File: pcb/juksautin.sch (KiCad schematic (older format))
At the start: 27 parts, among them J1 Screw_Terminal_01x09, J2 Serial_Debug, J3 AVR-ISP-6, J4 Conn_01x09, U1 SP3485EN, U2 SRV05-4, U3 R-78E5.0-0.5, U4 ATmega328P-AU, Y1 X322516MLB4SI

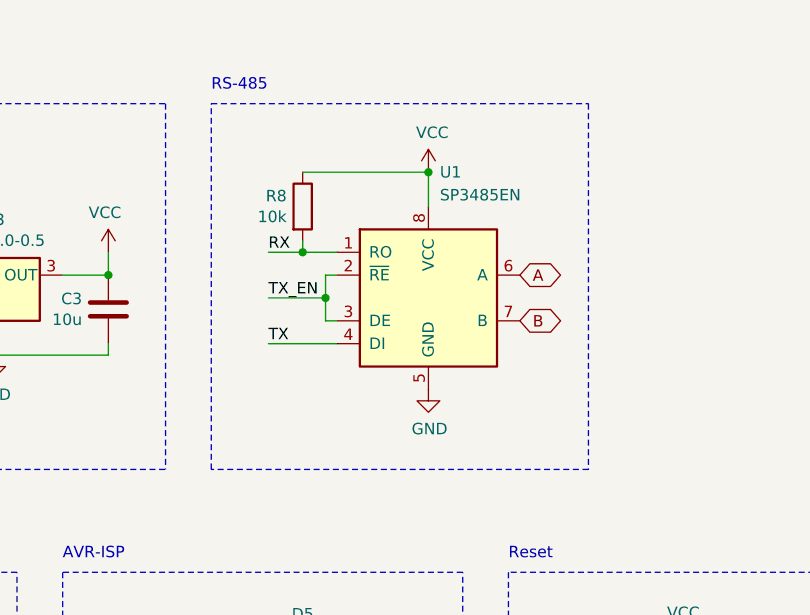
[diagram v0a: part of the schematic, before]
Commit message: pcb: Some changes. Don't remember anymore.
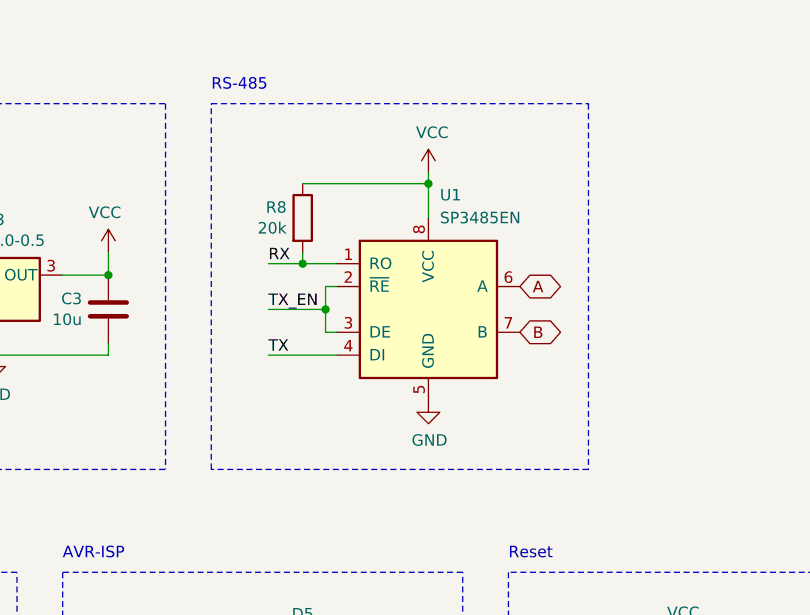
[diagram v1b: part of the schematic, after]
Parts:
- R8: value 10k -> 20k; LCSC C25804 -> C4184
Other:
- moved on the sheet: R8, U1
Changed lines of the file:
@@
 L power:GND #PWR0101
 U 1 1 60C357A5
-P 3750 2250
-F 0 "#PWR0101" H 3750 2000 50  0001 C CNN
-F 1 "GND" H 3755 2077 50  0000 C CNN
-F 2 "" H 3750 2250 50  0001 C CNN
-F 3 "" H 3750 2250 50  0001 C CNN
-	1    3750 2250
+P 3750 2300
+F 0 "#PWR0101" H 3750 2050 50  0001 C CNN
+F 1 "GND" H 3755 2127 50  0000 C CNN
+F 2 "" H 3750 2300 50  0001 C CNN
+F 3 "" H 3750 2300 50  0001 C CNN
+	1    3750 2300
 	1    0    0    -1
 $EndComp
@@
 LOW/HIGH/HI-Z\nemulates NTC
 Wire Wire Line
-	3350 1950 3300 1950
-Wire Wire Line
-	3350 1750 3300 1750
-Wire Wire Line
-	3300 1750 3300 1850
+	3350 2000 3300 2000
+Wire Wire Line
+	3350 1800 3300 1800
+Wire Wire Line
+	3300 1800 3300 1900
 Wire Wire Line
 	5650 5850 5650 5950
@@
 $EndComp
 Wire Wire Line
-	3750 1450 3750 1300
+	3750 1500 3750 1350
 $Comp
 L power:VCC #PWR0107
@@
 Text GLabel 1500 3900 3    50   UnSpc ~ 0
 K9
-Text GLabel 4150 1750 2    50   3State ~ 0
+Text GLabel 4150 1800 2    50   3State ~ 0
 A
-Text GLabel 4150 1950 2    50   3State ~ 0
+Text GLabel 4150 2000 2    50   3State ~ 0
 B
 Wire Wire Line
@@
 Text Notes 850  3000 0    50   ~ 0
 Screw terminal
-Connection ~ 3300 1850
-Wire Wire Line
-	3300 1850 3300 1950
+Connection ~ 3300 1900
+Wire Wire Line
+	3300 1900 3300 2000
 Wire Notes Line
 	2800 1000 4450 1000
@@
 L Interface_UART:SP3485EN U1
 U 1 1 60BB9B57
-P 3750 1850
+P 3750 1900
 F 0 "U1" H 3800 2400 50  0000 L CNN
 F 1 "SP3485EN" H 3800 2300 50  0000 L CNN
-F 2 "Package_SO:SOIC-8_3.9x4.9mm_P1.27mm" H 4800 1500 50  0001 C CIN
-F 3 "http://www.icbase.com/pdf/SPX/SPX00480106.pdf" H 3750 1850 50  0001 C CNN
-F 4 "C8963" H 3750 1850 50  0001 C CNN "LCSC"
-	1    3750 1850
+F 2 "Package_SO:SOIC-8_3.9x4.9mm_P1.27mm" H 4800 1550 50  0001 C CIN
+F 3 "http://www.icbase.com/pdf/SPX/SPX00480106.pdf" H 3750 1900 50  0001 C CNN
+F 4 "C8963" H 3750 1900 50  0001 C CNN "LCSC"
+	1    3750 1900
 	1    0    0    -1
 $EndComp
@@
 	1    0    0    -1
 $EndComp
-Text Label 3050 1650 0    50   ~ 0
+Text Label 3050 1700 0    50   ~ 0
 RX
 Wire Wire Line
-	3050 1650 3200 1650
-Text Label 3050 2050 0    50   ~ 0
+	3050 1700 3200 1700
+Text Label 3050 2100 0    50   ~ 0
 TX
 Wire Wire Line
-	3050 2050 3350 2050
+	3050 2100 3350 2100
 Text Label 9450 3250 0    50   ~ 0
 RX
@@
 Text Label 9450 3450 0    50   ~ 0
 TX_EN
-Text Label 3050 1850 0    50   ~ 0
+Text Label 3050 1900 0    50   ~ 0
 TX_EN
 Wire Wire Line
-	3050 1850 3300 1850
+	3050 1900 3300 1900
 Text Label 1150 5400 0    50   ~ 0
 PUMPFAIL_M
@@
 L Device:R R8
 U 1 1 60D023E7
-P 3200 1450
-F 0 "R8" H 3130 1496 50  0000 R CNN
-F 1 "10k" H 3130 1405 50  0000 R CNN
-F 2 "Resistor_SMD:R_0603_1608Metric" V 3130 1450 50  0001 C CNN
-F 3 "~" H 3200 1450 50  0001 C CNN
-F 4 "C25804" H 3200 1450 50  0001 C CNN "LCSC"
-	1    3200 1450
-	1    0    0    -1
-$EndComp
-Wire Wire Line
-	3200 1600 3200 1650
-Connection ~ 3200 1650
-Wire Wire Line
-	3200 1650 3350 1650
-Wire Wire Line
-	3200 1300 3750 1300
-Connection ~ 3750 1300
+P 3200 1500
+F 0 "R8" H 3130 1546 50  0000 R CNN
+F 1 "20k" H 3130 1455 50  0000 R CNN
+F 2 "Resistor_SMD:R_0603_1608Metric" V 3130 1500 50  0001 C CNN
+F 3 "~" H 3200 1500 50  0001 C CNN
+F 4 "C4184" H 3200 1500 50  0001 C CNN "LCSC"
+	1    3200 1500
+	1    0    0    -1
+$EndComp
+Wire Wire Line
+	3200 1650 3200 1700
+Connection ~ 3200 1700
+Wire Wire Line
+	3200 1700 3350 1700
+Wire Wire Line
+	3200 1350 3750 1350
+Connection ~ 3750 1350
+Wire Wire Line
+	3750 1300 3750 1350
 $EndSCHEMATC
